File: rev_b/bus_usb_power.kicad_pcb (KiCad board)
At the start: 2 copper layers, 100 x 50 mm, 27 parts, among them J1 TERMINATE_JUMPER, Q1 FQP47P06, Q2 FQP47P06, SW1 F-426-0020

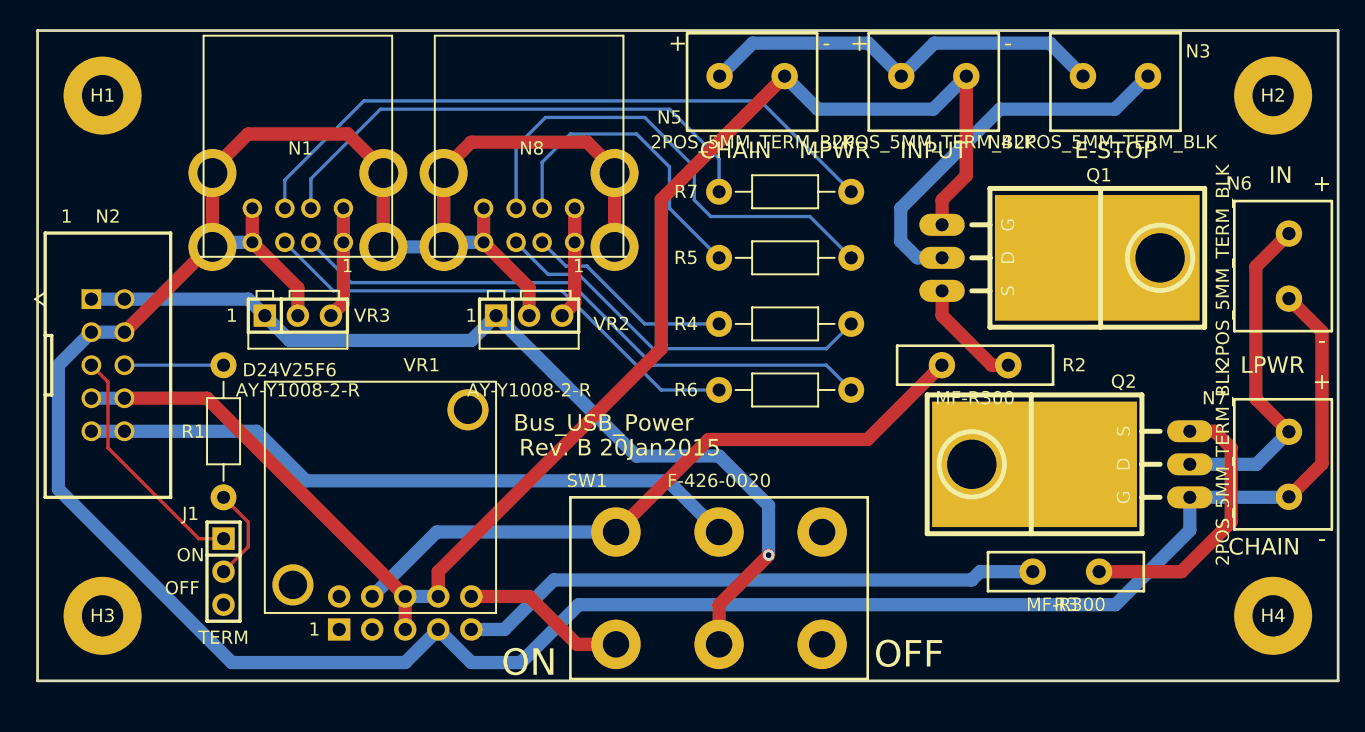
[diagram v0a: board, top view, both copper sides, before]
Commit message: Rev. B is looking pretty good.
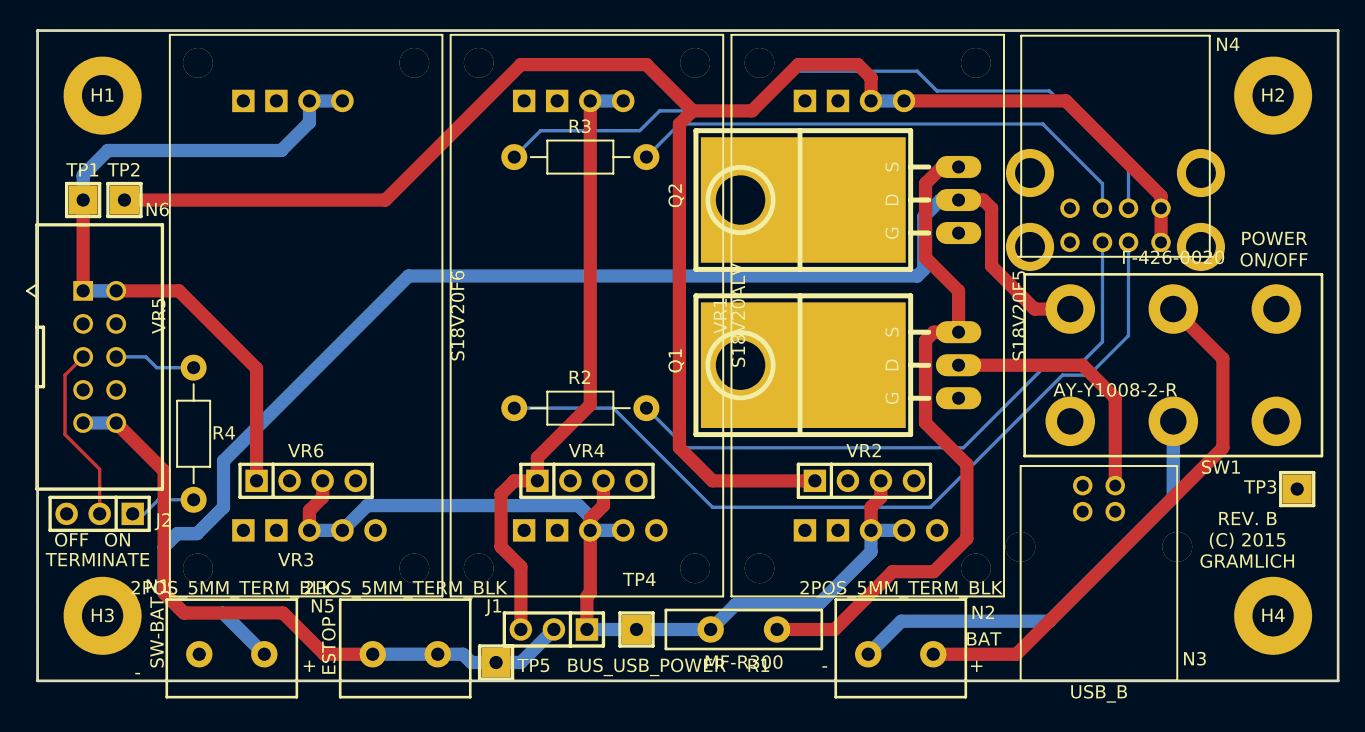
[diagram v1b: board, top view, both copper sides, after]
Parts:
- removed N7: 2POS_5MM_TERM_BLK, Bus_Usb_Power:5MM_TERMINAL_BLOCK_2_POS
- removed N8: AY-Y1008-2-R, Bus_Usb_Power:DUAL_USB_A
- removed R5, R6, R7: 200, Bus_Usb_Power:Resistor_Horizontal_400
- added J2: TERMINATE_JUMPER, Bus_Usb_Power:Pin_Header_Straight_1x03, F.Cu at (104.8, 137.2)
- added TP1: TEST_POINT, Bus_Usb_Power:Pin_Header_Straight_1x01, F.Cu at (103.5, 113.0)
- added TP2: TEST_POINT, Bus_Usb_Power:Pin_Header_Straight_1x01, F.Cu at (106.7, 113.0)
- added TP3: TEST_POINT, Bus_Usb_Power:Pin_Header_Straight_1x01, F.Cu at (196.8, 135.3)
- added TP4: TEST_POINT, Bus_Usb_Power:Pin_Header_Straight_1x01, F.Cu at (146.1, 146.1)
- added TP5: TEST_POINT, Bus_Usb_Power:Pin_Header_Straight_1x01, F.Cu at (135.3, 148.6)
- added VR4: S7V8A, Bus_Usb_Power:Pin_Header_Straight_1x04, F.Cu at (142.2, 134.6)
- added VR5: S18V20F6, Bus_Usb_Power:S18V20Fx, F.Cu at (120.7, 121.9)
- added VR6: S7V8A, Bus_Usb_Power:Pin_Header_Straight_1x04, F.Cu at (120.7, 134.6)
- J1: value TERMINATE_JUMPER -> POWER_SELECT
- N1: value AY-Y1008-2-R -> 2POS_5MM_TERM_BLK; footprint Bus_Usb_Power:DUAL_USB_A -> Bus_Usb_Power:5MM_TERMINAL_BLOCK_2_POS
- N2: value BUS_MASTER_HEADER -> 2POS_5MM_TERM_BLK; footprint Bus_Usb_Power:Pin_Header_Straight_2x05_Shrouded -> Bus_Usb_Power:5MM_TERMINAL_BLOCK_2_POS
- N3: value 2POS_5MM_TERM_BLK -> USB_B; footprint Bus_Usb_Power:5MM_TERMINAL_BLOCK_2_POS -> Bus_Usb_Power:USB_B
- N4: value 2POS_5MM_TERM_BLK -> AY-Y1008-2-R; footprint Bus_Usb_Power:5MM_TERMINAL_BLOCK_2_POS -> Bus_Usb_Power:DUAL_USB_A
- N6: value 2POS_5MM_TERM_BLK -> BUS_MASTER_HEADER; footprint Bus_Usb_Power:5MM_TERMINAL_BLOCK_2_POS -> Bus_Usb_Power:Pin_Header_Straight_2x05_Shrouded
- R1: value 120 1% -> MF-R300; footprint Bus_Usb_Power:Resistor_Horizontal_400 -> Bus_Usb_Power:MF_R300
- R2, R3: value MF-R300 -> 200; footprint Bus_Usb_Power:MF_R300 -> Bus_Usb_Power:Resistor_Horizontal_400
- R4: value 200 -> 120 1%
- VR1: value D24V25F6 -> S18V20F5; footprint Bus_Usb_Power:D24V25F6 -> Bus_Usb_Power:S18V20Fx
- VR2: value OKI-78SR-5/1.5-W36-C -> S7VVF5; footprint Bus_Usb_Power:OKI_DC_TO_DC_CONNECTOR -> Bus_Usb_Power:Pin_Header_Straight_1x04
- VR3: value OKI-78SR-5/1.5-W36-C -> S18V20ALV; footprint Bus_Usb_Power:OKI_DC_TO_DC_CONNECTOR -> Bus_Usb_Power:S18V20Fx
- moved N6 91.7 mm to (104.8, 125.1), turned to 270 degrees
- moved N2 64.9 mm to (166.4, 148.0), turned to 0 degrees
- moved N5 51.8 mm to (128.3, 148.0), turned to 0 degrees
- moved R3 49.1 mm to (141.7, 109.7), turned to 0 degrees
- moved R4 46.3 mm to (112.0, 131.0), turned to 270 degrees
- moved R1 42.8 mm to (154.3, 146.1), turned to 180 degrees
- moved VR1 40.0 mm to (163.8, 121.9), turned to 90 degrees
- moved SW1 38.9 mm to (187.3, 125.7)
- moved N3 36.2 mm to (181.6, 139.7), turned to 0 degrees
- moved N1 34.7 mm to (114.9, 148.0), turned to 0 degrees
- moved R2 30.5 mm to (141.7, 129.0), turned to 0 degrees
- moved VR2 28.7 mm to (163.6, 134.6)
- moved Q2 27.0 mm to (170.8, 113.0)
- moved J1 25.8 mm to (139.7, 146.1), turned to 180 degrees
- moved VR3 22.2 mm to (142.2, 121.9), turned to 90 degrees
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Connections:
- net /MPWR1 renamed /USB_5V_IN
- J1 pad 1: Net-(J1-Pad1) -> /FUSE_IN
- J1 pad 2: Net-(J1-Pad2) -> /BPWR2
- J1 pad 3: (no net) -> /BPWR1
- N1 pad 1: /USB2_5V -> /GND
- N1 pad 2: Net-(N1-Pad2) -> /BAT_SW
- N2 pad 1: /LPWR5 -> /BAT-
- N2 pad 2: /LPWR5 -> /BAT+
- N3 pad 2: /MPWR0 -> (no net)
- N4 pad 1: /MGND -> /USB_5V
- N4 pad 2: /MPWR0 -> Net-(N4-Pad2)
- N5 pad 1: /MGND -> /BPWR2
- N5 pad 2: /MPWR0 -> /BPWR2
- N6 pad 1: /LGND -> /LPWR
- N6 pad 2: /LPWR1 -> /LPWR
- Q1 pad G: /MGND -> /GND
- Q1 pad S: /MPWR2 -> /PWRCOM
- Q2 pad D: /LPWR1 -> /BAT_SW
- Q2 pad G: /LGND -> /GND
- Q2 pad S: /LPWR2 -> /PWRCOM
- R1 pad 1: Net-(J1-Pad2) -> /PWRCOM
- R1 pad 2: Net-(N2-Pad6) -> /FUSE_IN
- R2 pad 1: /MPWR2 -> Net-(N4-Pad2)
- R2 pad 2: /MPWR3 -> Net-(N4-Pad3)
- R3 pad 1: /LPWR2 -> Net-(N4-Pad6)
- R3 pad 2: /LPWR3 -> Net-(N4-Pad7)
- R4 pad 1: Net-(N8-Pad2) -> Net-(N6-Pad6)
- SW1 pad 1: /MPWR3 -> /BAT_SW
- SW1 pad 2: /MPWR4 -> /BAT+
- SW1 pad 4: /LPWR4 -> /GND
- SW1 pad 5: /LPWR5 -> /BAT-
- VR1 pad 1: (no net) -> /GND
- VR1 pad 10: /LPWR4 -> (no net)
- VR1 pad 2: (no net) -> /GND
- VR1 pad 3: (no net) -> /FUSE_IN
- VR1 pad 4: /MPWR3 -> /FUSE_IN
- VR1 pad 5: /MGND -> (no net)
- VR1 pad 6: /MGND -> /GND
- VR1 pad 7: /LGND -> /GND
- VR1 pad 8: /MGND -> /USB_5V
- VR1 pad 9: /LPWR3 -> /USB_5V
- VR2 pad 1: /LPWR5 -> /USB_5V
- VR2 pad 2: /LGND -> /GND
- VR2 pad 3: /USB1_5V -> /FUSE_IN
- VR3 pad 1: /LPWR5 -> /GND
- VR3 pad 2: /LGND -> /GND
- VR3 pad 3: /USB2_5V -> /FUSE_IN
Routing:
- net /LGND: track 235.0 -> 0.00 mm
- net /USB_5V: track 0.00 -> 133.5 mm
- net /MGND: track 114.8 -> 0.00 mm
- net /BAT_SW: track 0.00 -> 104.5 mm
- net /FUSE_IN: track 0.00 -> 75.1 mm
- net /LPWR5: track 72.5 -> 0.00 mm, vias 1 -> 0
- net Net-(N4-Pad2): track 0.00 -> 63.0 mm
- net /LPWR: track 0.00 -> 56.6 mm
- net Net-(N4-Pad6): track 0.00 -> 56.1 mm
- net /PWRCOM: track 0.00 -> 52.4 mm
- net /MPWR4: track 51.5 -> 0.00 mm
- net /MPWR3: track 51.2 -> 0.00 mm
- net Net-(N1-Pad7): track 51.1 -> 0.00 mm
- net /BPWR2: track 0.00 -> 50.4 mm
- net /BPWR1: track 0.00 -> 47.7 mm
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- added copper zone on B.Cu, net /GND
- added copper zone on F.Cu, net /GND
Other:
- board text added: "BAT"
- board text added: "BUS_USB_POWER"
- board text added: "ESTOP"
- board text added: "POWER ON/OFF"
- board text added: "REV. B (C) 2015 GRAMLICH"
- board text added: "SW-BAT"
- board text added: "TERMINATE"
- board text removed: "1"
- board text removed: "Bus USB Power Rev. B 20Jan2015 Copyright (c) 2015 by Wayne Gramlich"
- board text removed: "Bus_USB_Power"
- board text removed: "CHAIN"
- board text removed: "E-STOP"
- board text removed: "IN"
- board text removed: "INPUT"
- board text removed: "LPWR"
- board text removed: "MPWR"
- board text removed: "Rev. B 20Jan2015"
- board text removed: "TERM"
